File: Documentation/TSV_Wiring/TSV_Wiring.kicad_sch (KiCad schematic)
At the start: 24 parts, among them P1 SurLok, P2 SurLok, P3 SurLok, P4 SurLok, P5 SurLok, P6 SurLok, U1 Medusa, U10 GIGIVAC AIR, U11 GIGIVAC AIR, U12 BRB, U2 ElCon_Charger, U3 HV_distribution_enclosure, U4 Motor_Controler, U5 MRAX_228, U6 GIGVAC ROTARY HVD, U7 GIGIVAC AIR, U8 GIGIVAC AIR, U9 GIGVAC ROTARY HVD

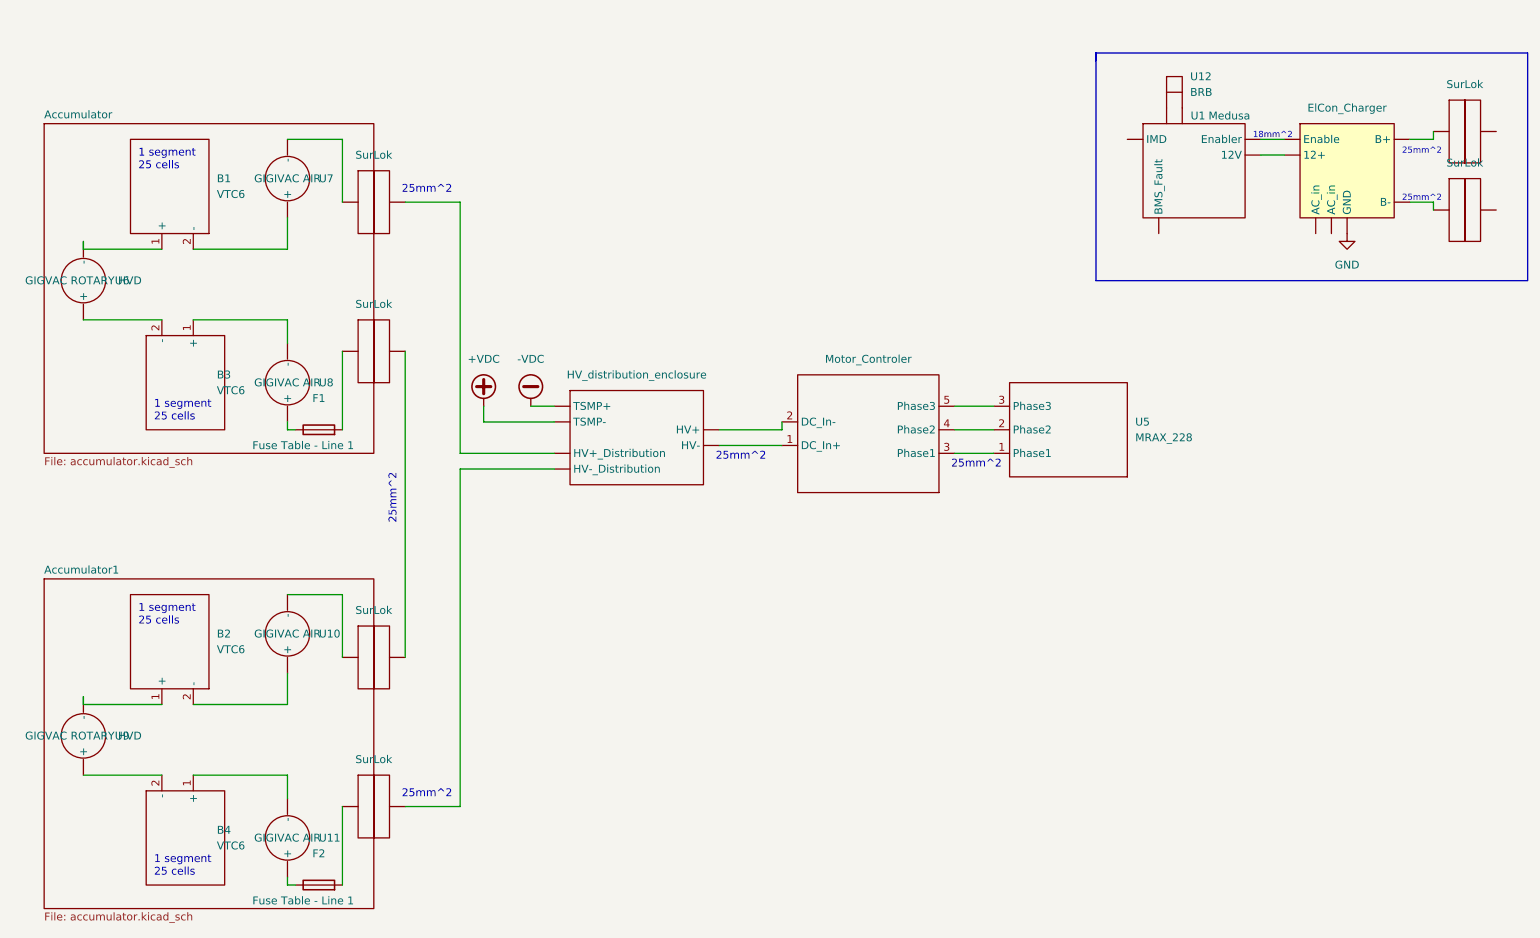
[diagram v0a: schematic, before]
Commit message: CleanSpeed
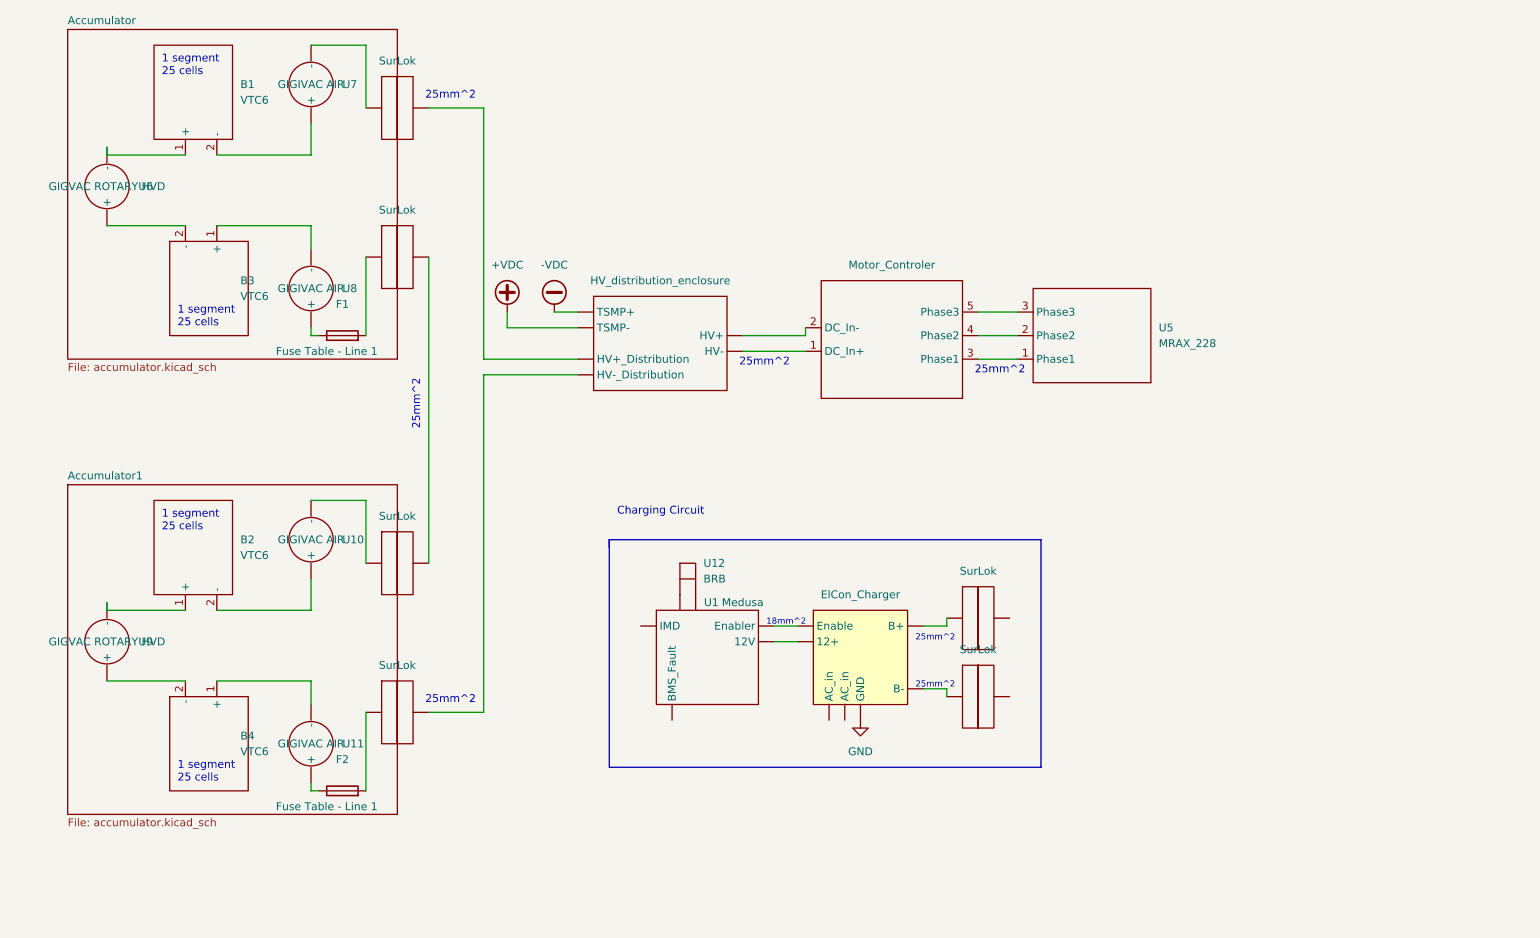
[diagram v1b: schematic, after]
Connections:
- net at P5.: now also U2. (GND)
- net at P1.: now also U7. (-); no longer U3. (TSMP-)
- net at U1. (IMD): now also U2. (GND); no longer U12.
- net at P6.: no longer U2. (GND)
- new net: P1., U3. (TSMP-)
- new net: U1. (IMD), U12.
- new net: U1. (IMD), U2. (GND)
- new net: P6., U2. (GND)
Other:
- note added: "Charging Circuit"
- title: TSV -> TSV Wiring
- moved on the sheet: B1, B2, B3, B4, F1, F2, U1, U10, U11, U12, U5, U6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
